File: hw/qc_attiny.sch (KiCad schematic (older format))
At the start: 14 parts, among them J1 USB_A, SW1 SW_DIP, SW2 SW_Push, U1 ATtiny84A-PU, U2 LM1117-3.3

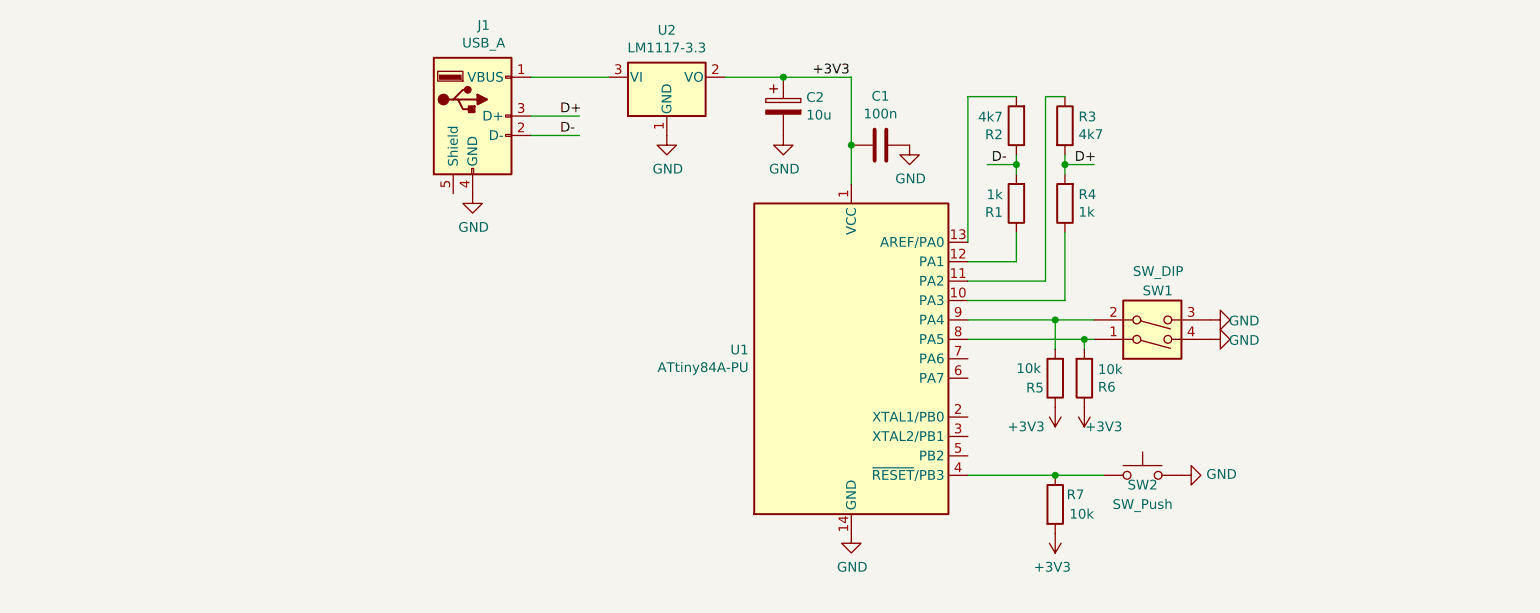
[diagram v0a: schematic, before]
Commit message: Update shematic
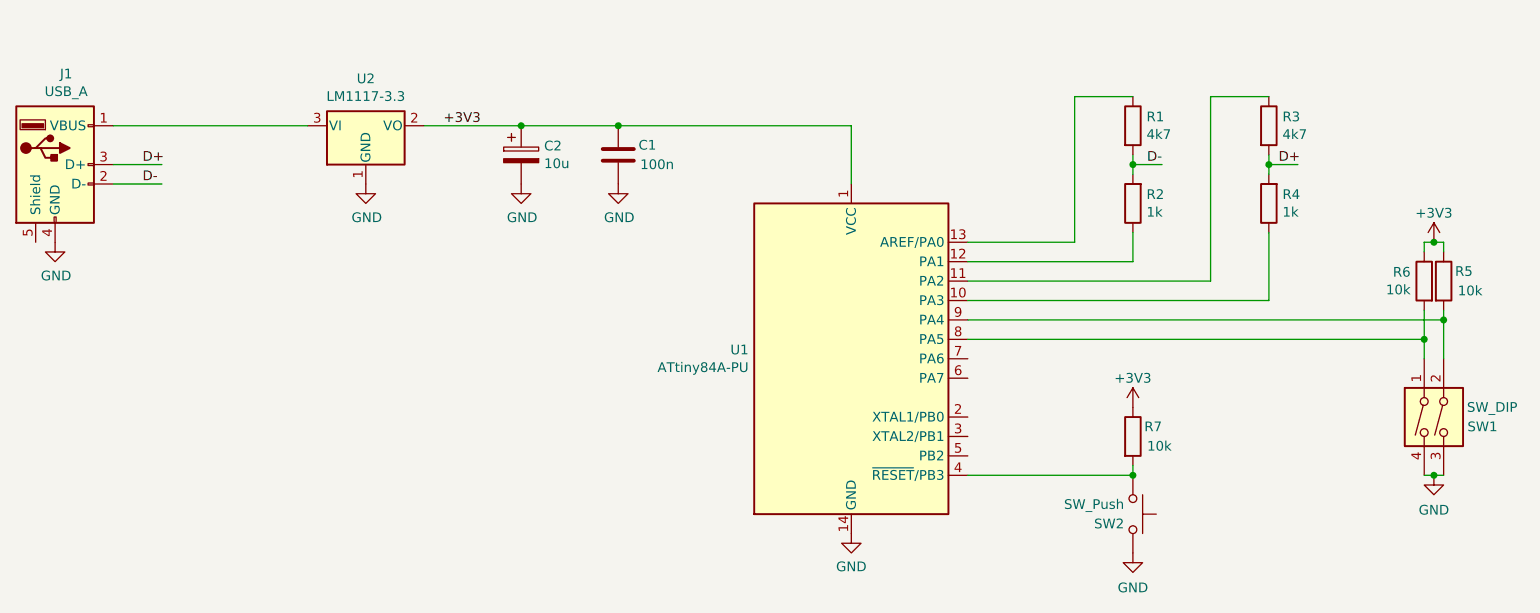
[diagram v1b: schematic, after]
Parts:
- R1: value 1k -> 4k7
- R2: value 4k7 -> 1k
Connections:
- wire segments 30 -> 37
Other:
- moved on the sheet: C1, C2, J1, R3, R4, R5, R6, R7, SW1, SW2, U2
